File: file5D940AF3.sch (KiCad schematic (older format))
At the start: 92 parts, among them CN1 KEYBOARD_20PIN_MALE, CN10 LED_CONNECTOR, CN2 USER_PORT_CON, CN3 CASSETTE_PORT_CON, CN4 SERIAL_BUS_CON, CN7 POWER_CON, CN8 CONTROL_PORT, CN9 CONTROL_PORT, Q1 2SC1815, Q2 2SC1815, Q3 TP298/2SD880, SW1 POWER_SWITCH, U1 CIA_U1, U2 CIA_U2, U20 556, U27 7408_U27, U28 4066_U28, U7 6510_MPU, U8 7406N

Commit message: oscillator
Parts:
- added C107, C108: 10uF, KU-14194HB-RevB-KiCad:CAP_P5.08mm, symbol Device:C_Small
- added C36, C68: .1, KU-14194HB-RevB-KiCad:CAP_P5.08mm, symbol Device:C_Small
- added C70: ~, KU-14194HB-RevB-KiCad:CAP_P5.08mm, symbol Device:C_Small
- added C86: ?, KU-14194HB-RevB-KiCad:CAP_P5.08mm, symbol Device:C_Small
- added FB16, FB17: FERRITE_NARROW, KU-14194HB-RevB-KiCad:FERRITE_BEAD_TH_P12.7mm, symbol KU-schematics-library:FERRITE_NARROW
- added R101: ?, KU-14194HB-RevB-KiCad:RESISTOR, symbol KU-schematics-library:R_US_CUSTOM
- added R26: 100, KU-14194HB-RevB-KiCad:RESISTOR, symbol KU-schematics-library:R_US_CUSTOM
- added U31: 74LS629N, symbol KU-schematics-library:74LS629N
- added U? (x11): GND_SMALL, symbol KU-14194HB-REV-B-KiCad-rescue:GND_SMALL-power
- added Y1: Crystal, symbol KU-schematics-library:Crystal
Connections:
- net labels added: +Vc, DOT_CLOCK
- wire segments 540 -> 578
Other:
- moved on the sheet: C105, C24, C39, R34, R36, R50, U20B, U8F

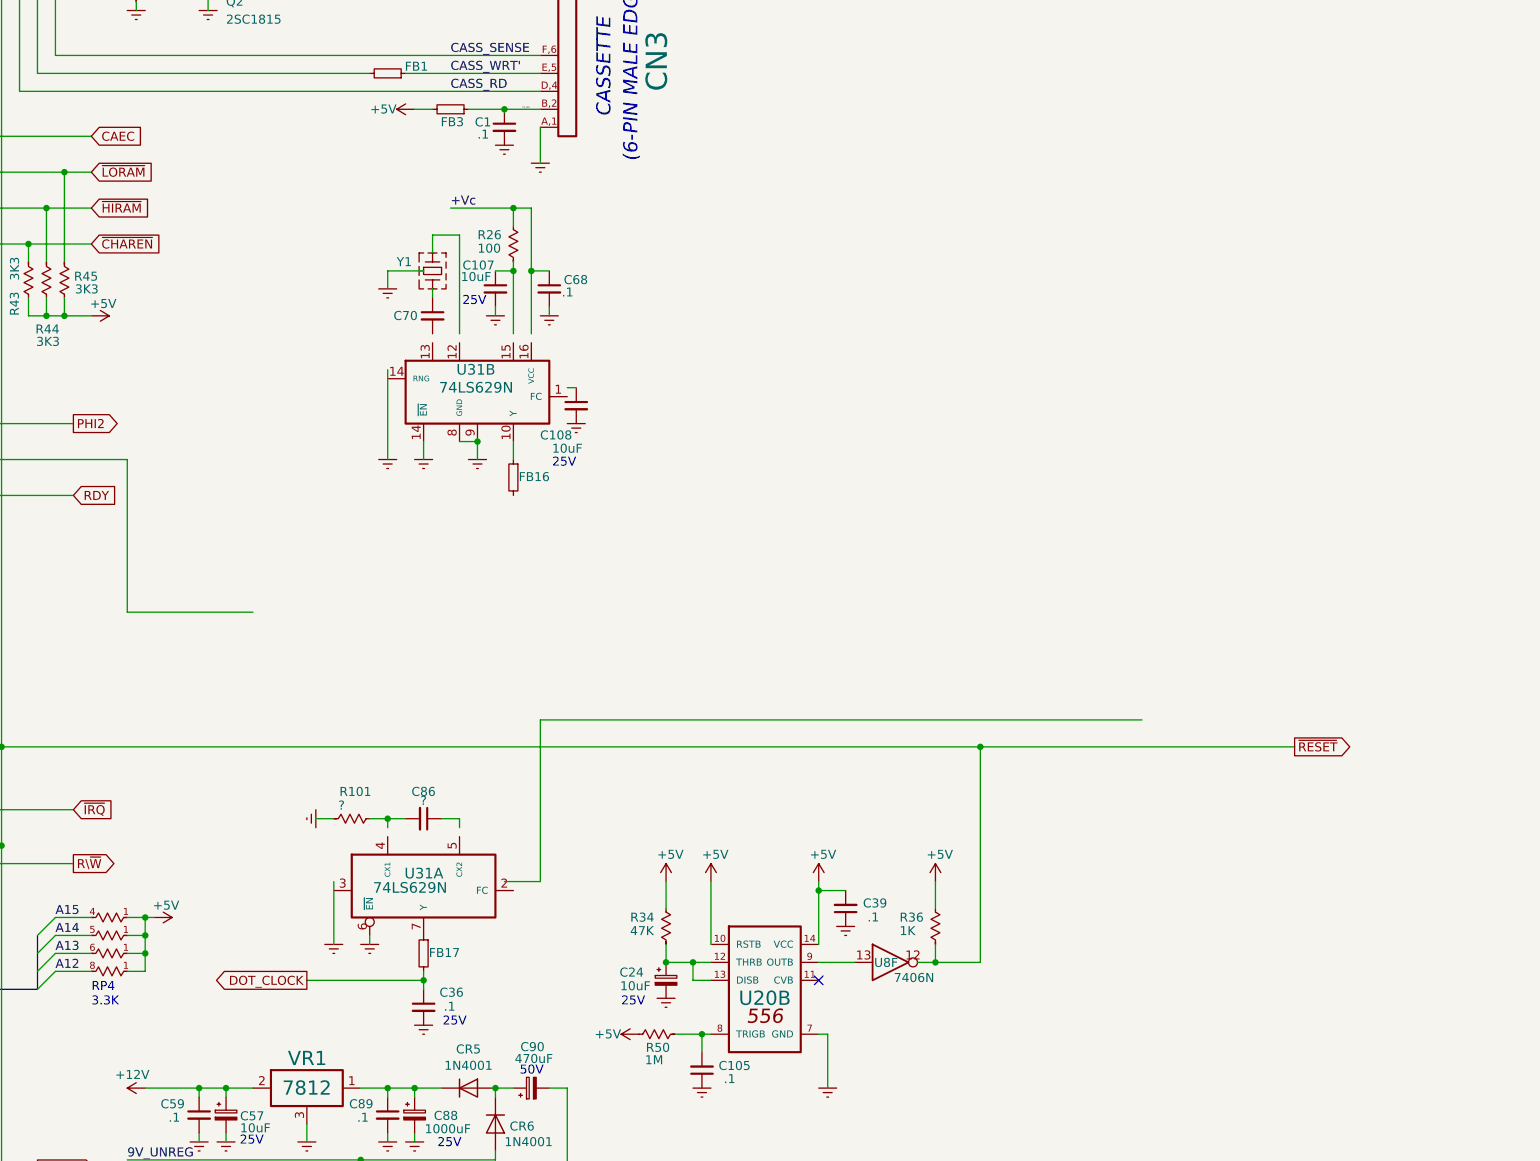
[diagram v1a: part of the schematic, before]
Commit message: Oscillator area
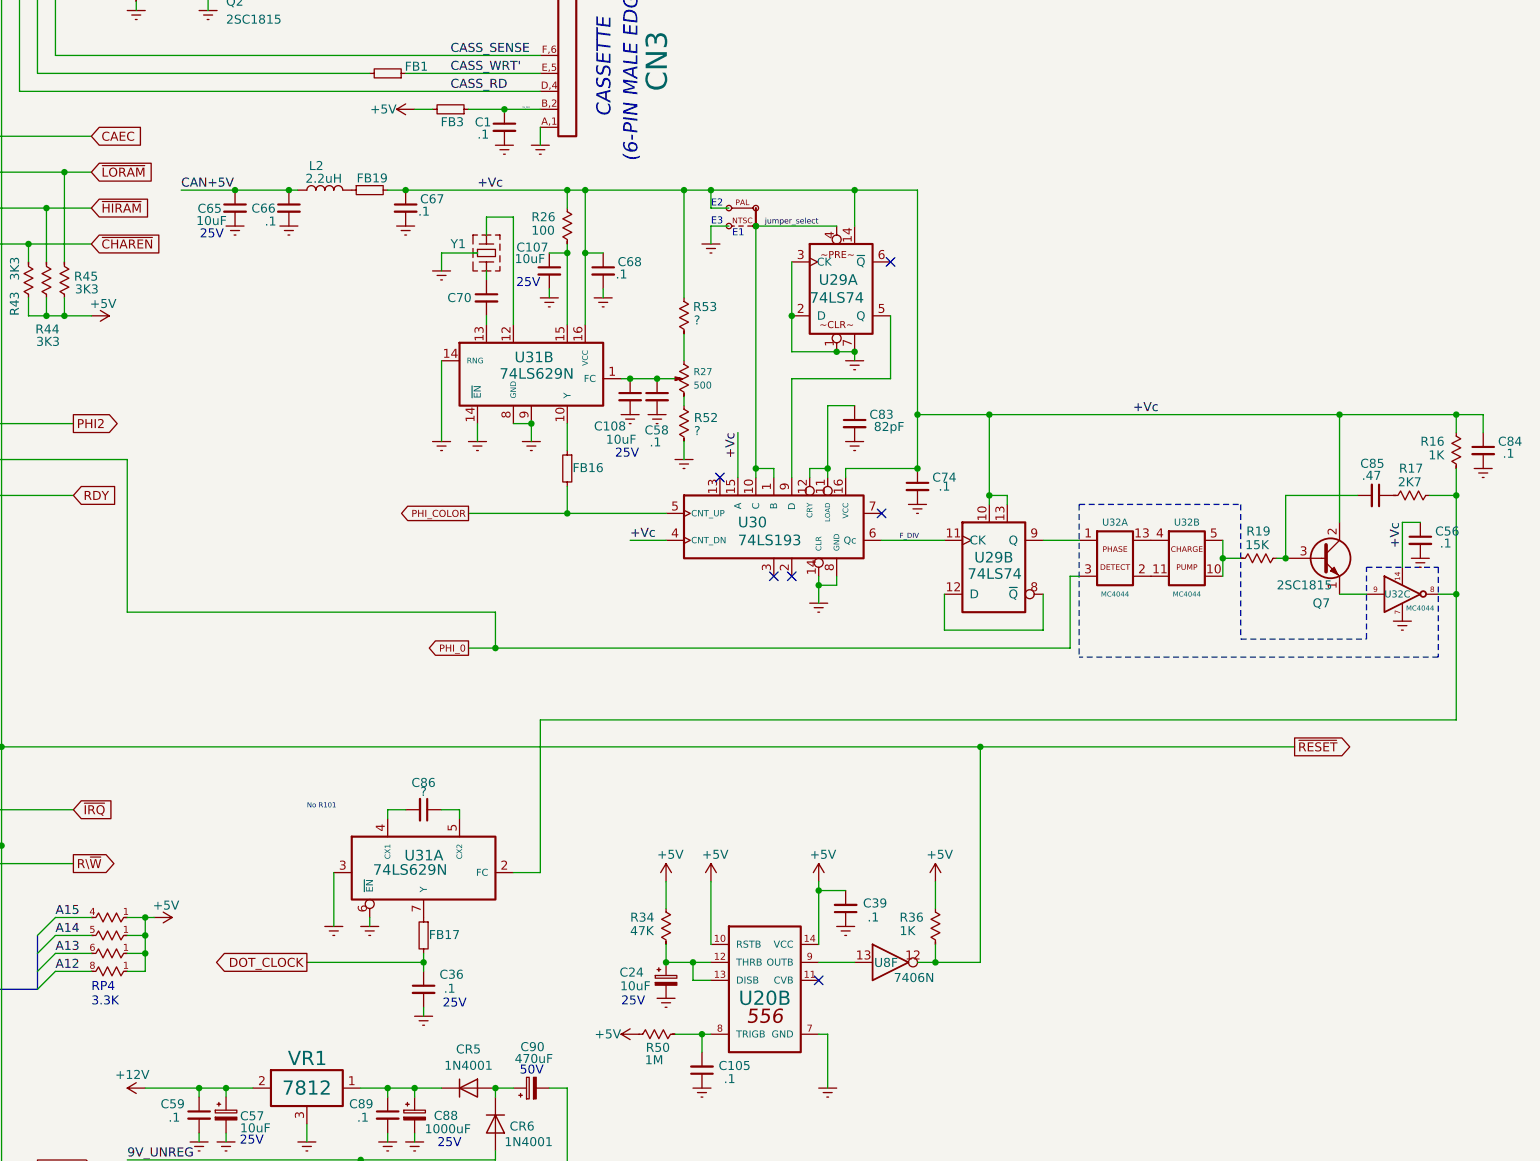
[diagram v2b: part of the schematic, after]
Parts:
- removed R101: ?, KU-14194HB-RevB-KiCad:RESISTOR, symbol KU-schematics-library:R_US_CUSTOM
- removed U? (x11): GND_SMALL, symbol KU-14194HB-REV-B-KiCad-rescue:GND_SMALL-power
- added C56, C58, C66, C67, C74, C84: .1, KU-14194HB-RevB-KiCad:CAP_P5.08mm, symbol Device:C_Small
- added C65: 10uF, KU-14194HB-RevB-KiCad:CAP_ELYT_RADIAL_P2.54mm, symbol Device:C_Small
- added C83: 82pF, KU-14194HB-RevB-KiCad:RESISTOR, symbol Device:C_Small
- added C85: .47, KU-14194HB-RevB-KiCad:CAP_P5.08mm, symbol Device:C_Small
- added E1: JUMPER_WIRE, KU-14194HB-RevB-KiCad:JUMPER_WIRE, symbol KU-schematics-library:JUMPER_WIRE
- added FB19: FERRITE_NARROW, KU-14194HB-RevB-KiCad:FERRITE_BEAD_TH_P12.7mm, symbol KU-schematics-library:FERRITE_NARROW
- added L2: 2.2uH, symbol Device:L
- added Q7: 2SC1815, KU-14194HB-RevB-KiCad:Q_NPN_ECB, symbol Transistor_BJT:2SC1815
- added R16: 1K, KU-14194HB-RevB-KiCad:RESISTOR, symbol KU-schematics-library:R_US_CUSTOM
- added R17: 2K7, KU-14194HB-RevB-KiCad:RESISTOR, symbol KU-schematics-library:R_US_CUSTOM
- added R19: 15K, KU-14194HB-RevB-KiCad:RESISTOR, symbol KU-schematics-library:R_US_CUSTOM
- added R27: 500, KU-14194HB-RevB-KiCad:POTMETER, symbol KU-schematics-library:R_POTMETER_US
- added R52, R53: ?, KU-14194HB-RevB-KiCad:RESISTOR, symbol KU-schematics-library:R_US_CUSTOM
- added U29: 74LS74, KU-14194HB-RevB-KiCad:DIP14, symbol KU-schematics-library:74LS74
- added U30: 74LS193, KU-14194HB-RevB-KiCad:DIP16, symbol KU-schematics-library:74LS193
- added U32: MC4044, KU-14194HB-RevB-KiCad:DIP14, symbol KU-schematics-library:MC4044
- C107, C108: footprint KU-14194HB-RevB-KiCad:CAP_P5.08mm -> KU-14194HB-RevB-KiCad:CAP_ELYT_RADIAL_P2.54mm
- C36, C70, C86: footprint KU-14194HB-RevB-KiCad:CAP_P5.08mm -> KU-14194HB-RevB-KiCad:RESISTOR
- U31: footprint (none) -> KU-14194HB-RevB-KiCad:DIP16
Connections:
- net +Vc: now also U31.16 (VCC), C56.1, C67.1, C74.1, C84.1, E1.1, FB19.2, Q7.2 (C), R16.1, R53.1, U29.10, U29.13, U29.14, U30.15 (A), U30.16 (VCC), U30.4 (CNT_DN), U32.14
- net CAN+5V: now also C65.1, C66.1, L2.1
- net Earth: now also U31.3, C56.2, C58.2, C65.2, C66.2, C67.2, C74.2, C83.2, C84.2, E1.2, R52.2, U29.1, U29.2 (D), U29.3 (CK), U29.7, U30.14 (CLR), U30.8 (GND), U32.7
- net PHI_0: now reaches U7.1 (PH0IN)
- net PHI_0: now also U32.3
- net at U31.2 (FC): now also R16.2, R17.1, U32.8
- net at U31.4 (CX1): now also C86.2
- net at U31.5 (CX2): now also C86.1
- net at U31.1 (FC): now also C108.1, C58.1, R27.3
- net at U31.12: now also Y1.1
- net at U31.13: now also C70.2
- net at U31.15: now also C107.1, R26.2
- net PHI_COLOR: now reaches FB16.2
- net PHI_COLOR: now also U30.5 (CNT_UP)
- new net: R27.1, R53.2
- new net: R27.2, R52.1
- new net: FB19.1, L2.2
- new net: Q7.1 (E), U32.9
- new net: C85.2, Q7.3 (B), R19.1
- new net: C83.1, U30.11 (LOAD), U30.12 (CRY)
- new net: U29.5 (Q), U30.9 (D)
- new net: R19.2, U32.10, U32.5
- new net: U29.12 (D), U29.8 (~Q~)
- new net: U29.9 (Q), U32.1
- new net: C85.1, R17.2
- new net: U32.13, U32.4
- new net: U32.11, U32.2
- new net F_DIV: U29.11 (CK), U30.6 (Qc)
- new net jumper_select: E1.C, U29.4, U30.1 (B), U30.10 (C)
- no-connect marks 3 -> 8
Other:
- note added: "E1"
- note added: "E2"
- note added: "E3"
- note added: "No R101"
- moved on the sheet: C107, C108, C36, C68, C70, C86, FB16, FB17, R26, U31A, U31B, Y1
